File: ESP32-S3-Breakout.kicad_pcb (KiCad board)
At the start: 4 copper layers, 29 x 54.4 mm, 34 parts, among them J1 USB_C_Receptacle_USB2.0, J2 USB_C_Receptacle_USB2.0, J3 Conn_01x21, J4 Conn_01x21, Q1 Q_NPN_BCE, Q2 Q_NPN_BCE, SW1 SW_Push, SW2 SW_Push, U1 USBLC6-2SC6, U2 USBLC6-2SC6, U3 ESP32-S3-WROOM, U4 CH340C, U5 XC6210B332MR, Y1 32.768kHz

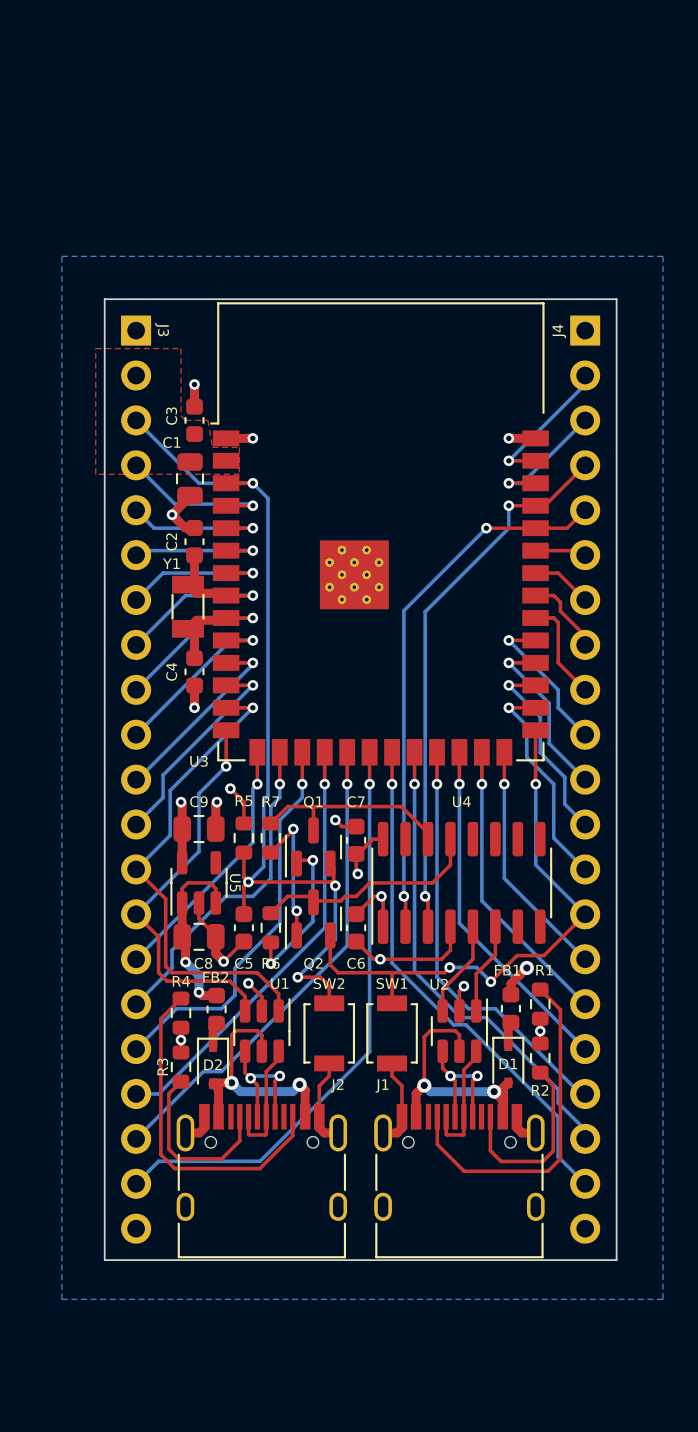
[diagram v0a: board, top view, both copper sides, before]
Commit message: initial group of modifications.
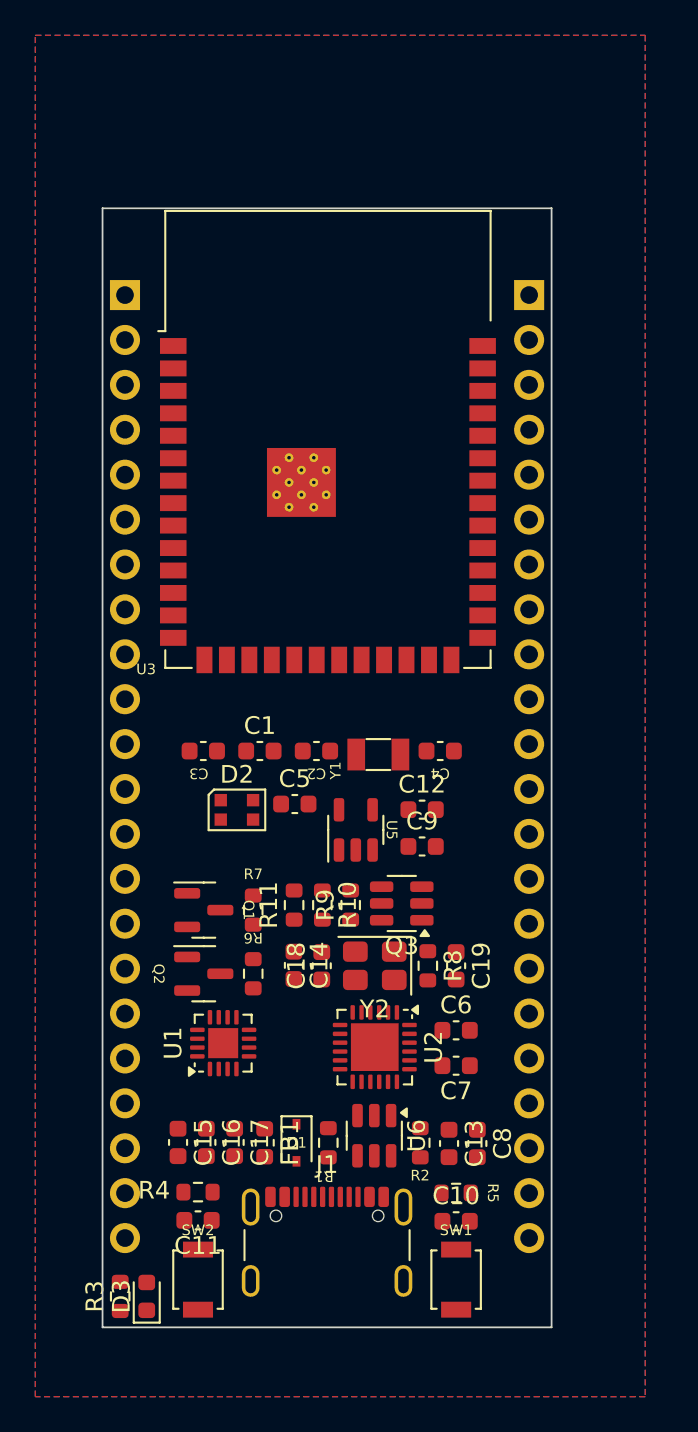
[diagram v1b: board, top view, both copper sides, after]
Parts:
- removed FB2: 500mA?, Inductor_SMD:L_0603_1608Metric
- removed J4: Conn_01x21, Connector_PinHeader_2.54mm:PinHeader_1x21_P2.54mm_Vertical
- removed U4: CH340C, Package_SO:SOIC-16_3.9x9.9mm_P1.27mm
- added C10: 4.7uF, Capacitor_SMD:C_0603_1608Metric, F.Cu at (94.3, 126.6)
- added C11: 1uF, Capacitor_SMD:C_0603_1608Metric, F.Cu at (79.7, 126.5)
- added C12: 10uF, Capacitor_SMD:C_0603_1608Metric, F.Cu at (92.4, 103.3)
- added C13: 10uF, Capacitor_SMD:C_0603_1608Metric, F.Cu at (93.9, 122.2)
- added C14: 10uF, Capacitor_SMD:C_0603_1608Metric, F.Cu at (85.1, 112.1)
- added C15: 100nF, Capacitor_SMD:C_0603_1608Metric, F.Cu at (78.6, 122.1)
- added C16: 100nF, Capacitor_SMD:C_0603_1608Metric, F.Cu at (80.2, 122.1)
- added C17: 100nF, Capacitor_SMD:C_0603_1608Metric, F.Cu at (81.8, 122.1)
- added C18: 15pF, Capacitor_SMD:C_0603_1608Metric, F.Cu at (86.7, 112.1)
- added C19: 15pF, Capacitor_SMD:C_0603_1608Metric, F.Cu at (94.3, 112.1)
- added D3: LED, LED_SMD:LED_0603_1608Metric, F.Cu at (76.8, 130.8)
- added Q3: FDC6330L, Package_TO_SOT_SMD:TSOT-23-6, F.Cu at (91.2, 108.6)
- added R10: 100k, Resistor_SMD:R_0603_1608Metric, F.Cu at (86.7, 108.7)
- added R11: 100, Resistor_SMD:R_0603_1608Metric, F.Cu at (85.1, 108.7)
- added R8: 1k, Resistor_SMD:R_0603_1608Metric, F.Cu at (92.7, 112.1)
- added R9: 100k, Resistor_SMD:R_0603_1608Metric, F.Cu at (88.3, 108.7)
- added U6: USBLC6-2SC6, Package_TO_SOT_SMD:SOT-23-6, F.Cu at (89.7, 121.7)
- added Y2: 12Mhz, Crystal:Crystal_SMD_SeikoEpson_TSX3225-4Pin_3.2x2.5mm, F.Cu at (89.7, 112.1)
- C1: value 22u -> 22uF; footprint Capacitor_SMD:C_0805_2012Metric -> Capacitor_SMD:C_0603_1608Metric
- C2, C4: value 18p -> 15pF
- C3: value 0.1u -> 100nF
- C5: value 1u -> 100nF
- C6, C7: value 0.1u -> 1uF
- C8, C9: value 1u -> 1uF; footprint Capacitor_SMD:C_0805_2012Metric -> Capacitor_SMD:C_0603_1608Metric
- D2: value 1N5819WS -> WS2812B-2020; footprint Diode_SMD:D_SOD-323 -> LED_SMD:LED_WS2812B-2020_PLCC4_2.0x2.0mm
- FB1: value 500mA? -> 500mA; footprint Inductor_SMD:L_0603_1608Metric -> Fuse:Fuse_0603_1608Metric
- J1: value USB_C_Receptacle_USB2.0 -> USB_TYPE_C_16PIN; footprint Connector_USB:USB_C_Receptacle_HRO_TYPE-C-31-M-12 -> Connector_USB:USB_C_Receptacle_GCT_USB4105-xx-A_16P_TopMnt_Horizontal
- J2: value USB_C_Receptacle_USB2.0 -> Conn_01x22; footprint Connector_USB:USB_C_Receptacle_HRO_TYPE-C-31-M-12 -> Connector_PinHeader_2.54mm:PinHeader_1x22_P2.54mm_Vertical; moved to B.Cu
- J3: value Conn_01x21 -> Conn_01x22; footprint Connector_PinHeader_2.54mm:PinHeader_1x21_P2.54mm_Vertical -> Connector_PinHeader_2.54mm:PinHeader_1x22_P2.54mm_Vertical
- Q1, Q2: value Q_NPN_BCE -> S8050
- R3: value 5.1k -> 1k
- R4: value 5.1k -> 10k
- SW1: value SW_Push -> RESET
- SW2: value SW_Push -> BOOT
- U1: value USBLC6-2SC6 -> CH343P; footprint Package_TO_SOT_SMD:SOT-23-6 -> Package_DFN_QFN:QFN-16-1EP_3x3mm_P0.5mm_EP1.7x1.7mm
- U2: value USBLC6-2SC6 -> CH334F; footprint Package_TO_SOT_SMD:SOT-23-6 -> Package_DFN_QFN:QFN-24-1EP_4x4mm_P0.5mm_EP2.7x2.7mm
- U3: value ESP32-S3-WROOM -> ESP32-S3-WROOM-1-N16R8
- moved J2 51.1 mm to (75.6, 74.2), turned to 180 degrees
- moved R5 23.4 mm to (94.3, 125.0), turned to 180 degrees
- moved J3 22.3 mm to (98.4, 74.2)
- moved C8 19.6 mm to (95.5, 122.2), turned to -90 degrees
- moved C3 18.7 mm to (80.0, 100.0), turned to 180 degrees
- moved C1 15.9 mm to (83.2, 100.0), turned to 0 degrees
- moved FB1 15.9 mm to (83.5, 122.1), turned to -90 degrees
- moved SW2 15.8 mm to (79.7, 129.9)
- moved C4 14.6 mm to (93.4, 100.0), turned to 0 degrees
- moved D2 14.5 mm to (81.9, 103.3), turned to 0 degrees
- moved SW1 14.4 mm to (94.3, 129.9)
- moved R1 14.3 mm to (87.1, 122.1), turned to 90 degrees
- moved C7 13.9 mm to (94.3, 117.8), turned to 180 degrees
- moved C2 13.7 mm to (86.4, 100.0), turned to 0 degrees
- moved Y1 13.6 mm to (89.9, 100.2), turned to 0 degrees
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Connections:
- net /CC1_1 renamed /ESP32-S3/CC1_1
- net /CC2_1 renamed /ESP32-S3/CC2_1
- C1 pad 1: +3V3 -> +3.3V
- C2 pad 2: /IO15 -> /GPIO15
- C3 pad 1: +3V3 -> +3.3V
- C4 pad 1: /IO16 -> /GPIO16
- C5 pad 1: /EN -> +3.3V
- C6 pad 1: +3V3 -> /ESP32-S3/3.3VUSB
- C7 pad 1: +3V3 -> GND
- C7 pad 2: GND -> /ESP32-S3/3.3VUSB
- C9 pad 1: +3V3 -> +3.3V
- D1 pad 2: /VBUS1 -> /ESP32-S3/VBUS
- D2 pad 1: Net-(D2-Pad1) -> /LED_OUT
- D2 pad 2: /VBUS2 -> GND
- J1 pad A4: /VBUS1 -> /ESP32-S3/VBUS
- J1 pad A6: /USB_UART_D+ -> /ESP32-S3/USB_D+
- J1 pad A7: /USB_UART_D- -> /ESP32-S3/USB_D-
- J1 pad A9: /VBUS1 -> /ESP32-S3/VBUS
- J1 pad B4: /VBUS1 -> /ESP32-S3/VBUS
- J1 pad B6: /USB_UART_D+ -> /ESP32-S3/USB_D+
- J1 pad B7: /USB_UART_D- -> /ESP32-S3/USB_D-
- J1 pad B9: /VBUS1 -> /ESP32-S3/VBUS
- J3 pad 10: /IO17 -> /GPIO38
- J3 pad 11: /IO18 -> /GPIO37
- J3 pad 12: /IO8 -> /GPIO36
- J3 pad 13: /IO19 -> /GPIO35
- J3 pad 14: /IO20 -> /GPIO0
- J3 pad 15: /IO3 -> /GPIO45
- J3 pad 16: /IO46 -> /GPIO48
- J3 pad 17: /IO9 -> /GPIO47
- J3 pad 18: /IO10 -> /GPIO21
- J3 pad 19: /IO11 -> /ESP_USB+
- J3 pad 2: +3V3 -> /ESP_TX0
- J3 pad 20: /IO12 -> /ESP_USB-
- J3 pad 21: +5V -> GND
- J3 pad 3: /EN -> /ESP_RX0
- J3 pad 4: /IO4 -> /GPIO1
- J3 pad 5: /IO5 -> /GPIO2
- J3 pad 6: /IO6 -> /GPIO42
- J3 pad 7: /IO7 -> /GPIO41
- J3 pad 8: /IO15 -> /GPIO40
- J3 pad 9: /IO16 -> /GPIO39
- Q1 pad 2: /EN -> /ENABLE
- Q1 pad 3: /RTS -> /ESP32-S3/RTS
- Q2 pad 2: /IO0 -> /GPIO0
- Q2 pad 3: /DTR -> /ESP32-S3/DTR
- R3 pad 1: /CC1_2 -> +3.3V
- R3 pad 2: GND -> Net-(D3-A)
- R4 pad 1: /CC2_2 -> /GPIO0
- R4 pad 2: GND -> +3.3V
- R5 pad 1: +3V3 -> +3.3V
- R5 pad 2: /EN -> /ENABLE
- R6 pad 1: /DTR -> /ESP32-S3/DTR
- R7 pad 1: /RTS -> /ESP32-S3/RTS
- SW1 pad 1: /IO0 -> /ENABLE
- SW2 pad 1: /EN -> /GPIO0
- U1 pad 1: /IO19 -> /ESP32-S3/3.3VUSB
- U1 pad 3: /IO20 -> /ESP32-S3/3.3VUSB
- U1 pad 4: /USB_D+ -> /ESP_RX0
- U1 pad 5: /VBUS2 -> /ESP_TX0
- U1 pad 6: /USB_D- -> /ESP32-S3/3.3VUSB
- U2 pad 1: /UART_D- -> unconnected-(U2-~{OVCUR}-Pad1)
- U2 pad 2: GND -> unconnected-(U2-Pad2)
- U2 pad 3: /UART_D+ -> Net-(U2-XOUT)
- U2 pad 4: /USB_UART_D+ -> Net-(U2-XIN)
- U2 pad 5: /VBUS1 -> unconnected-(U2-D-4-Pad5)
- U2 pad 6: /USB_UART_D- -> unconnected-(U2-D+4-Pad6)
- U3 pad 10: /IO17 -> /GPIO17
- U3 pad 11: /IO18 -> /GPIO18
- U3 pad 12: /IO8 -> /GPIO8
- U3 pad 13: /IO19 -> /ESP_USB-
- U3 pad 14: /IO20 -> /ESP_USB+
- U3 pad 15: /IO3 -> /GPIO3
- U3 pad 16: /IO46 -> /GPIO46
- U3 pad 17: /IO9 -> /GPIO9
- U3 pad 18: /IO10 -> /GPIO10
- U3 pad 19: /IO11 -> /GPIO11
- U3 pad 2: +3V3 -> +3.3V
- U3 pad 20: /IO12 -> /GPIO12
- U3 pad 21: /IO13 -> /GPIO13
- U3 pad 22: /IO14 -> /GPIO14
- U3 pad 23: /IO21 -> /GPIO21
- U3 pad 24: /IO47 -> /GPIO47
- U3 pad 25: /IO48 -> /GPIO48
- U3 pad 26: /IO45 -> /GPIO45
- U3 pad 27: /IO0 -> /GPIO0
- U3 pad 28: /IO35 -> /GPIO35
- U3 pad 29: /IO36 -> /GPIO36
- U3 pad 3: /EN -> /ENABLE
- U3 pad 30: /IO37 -> /GPIO37
- U3 pad 31: /IO38 -> /GPIO38
- U3 pad 32: /IO39 -> /GPIO39
- U3 pad 33: /IO40 -> /GPIO40
- U3 pad 34: /IO41 -> /GPIO41
- U3 pad 35: /IO42 -> /GPIO42
- U3 pad 36: /RXD0 -> /ESP_RX0
- U3 pad 37: /TXD0 -> /ESP_TX0
- U3 pad 38: /IO2 -> /GPIO2
- U3 pad 39: /IO1 -> /GPIO1
- U3 pad 4: /IO4 -> /GPIO4
- U3 pad 5: /IO5 -> /GPIO5
- U3 pad 6: /IO6 -> /GPIO6
- U3 pad 7: /IO7 -> /GPIO7
- U3 pad 8: /IO15 -> /GPIO15
- U3 pad 9: /IO16 -> /GPIO16
- U5 pad 5: +3V3 -> +3.3V
- Y1 pad 1: /IO16 -> /GPIO16
- Y1 pad 2: /IO15 -> /GPIO15
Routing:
- net /EN: track 52.0 -> 0.00 mm, vias 4 -> 0
- net GND: track 42.0 -> 0.00 mm, vias 13 -> 0
- net /IO12: track 33.2 -> 0.00 mm, vias 1 -> 0
- net /IO0: track 31.6 -> 0.00 mm, vias 3 -> 0
- net /TXD0: track 31.1 -> 0.00 mm, vias 2 -> 0
- net /RXD0: track 30.5 -> 0.00 mm, vias 2 -> 0
- net /IO13: track 29.3 -> 0.00 mm, vias 1 -> 0
- net /IO19: track 27.6 -> 0.00 mm, vias 1 -> 0
- net /IO11: track 27.4 -> 0.00 mm, vias 1 -> 0
- net /IO14: track 26.7 -> 0.00 mm, vias 1 -> 0
- net /IO10: track 24.5 -> 0.00 mm, vias 1 -> 0
- net /IO21: track 23.8 -> 0.00 mm, vias 1 -> 0
- net /IO20: track 22.6 -> 0.00 mm, vias 1 -> 0
- net /IO9: track 22.2 -> 0.00 mm, vias 1 -> 0
- net /IO47: track 19.7 -> 0.00 mm, vias 1 -> 0
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- added copper zone on B.Cu, net GND
- added copper zone on F.Cu, net GND
- added copper zone on In2.Cu, net GND
- removed copper zone on F.Cu, net +3V3
- removed copper zone on In2.Cu, net +3V3
- removed copper zone on B.Cu, net +5V
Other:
- board size 29 x 54.4 mm -> 25.4 x 63.3 mm
- board text removed: "3V3"
- board text removed: "5V"
- board text removed: "EN"
- board text removed: "ESP32-S3 DEV Module"
- board text removed: "GND"
- board text removed: "IO0"
- board text removed: "IO1"
- board text removed: "IO10"
- board text removed: "IO11"
- board text removed: "IO12"
- board text removed: "IO13"
- board text removed: "IO14"
- board text removed: "IO15"
- board text removed: "IO16"
- board text removed: "IO17"
- board text removed: "IO18"
- board text removed: "IO19"
- board text removed: "IO2"
- board text removed: "IO20"
- board text removed: "IO21"
- board text removed: "IO3"
- board text removed: "IO35"
- board text removed: "IO36"
- board text removed: "IO37"
- board text removed: "IO38"
- board text removed: "IO39"
- board text removed: "IO4"
- board text removed: "IO40"
- board text removed: "IO41"
- board text removed: "IO42"
- board text removed: "IO45"
- board text removed: "IO46"
- board text removed: "IO47"
- board text removed: "IO48"
- board text removed: "IO5"
- board text removed: "IO6"
- board text removed: "IO7"
- board text removed: "IO8"
- board text removed: "IO9"
- board text removed: "RXD0"
- board text removed: "Rev 1 12/2022"
- board text removed: "TXD0"
- board text removed: "UART"
- board text removed: "USB"
